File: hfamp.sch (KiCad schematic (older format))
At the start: 20 parts, among them K1 CONN_3, P1 CONN_2, Q1 DARL_N, U1 7805

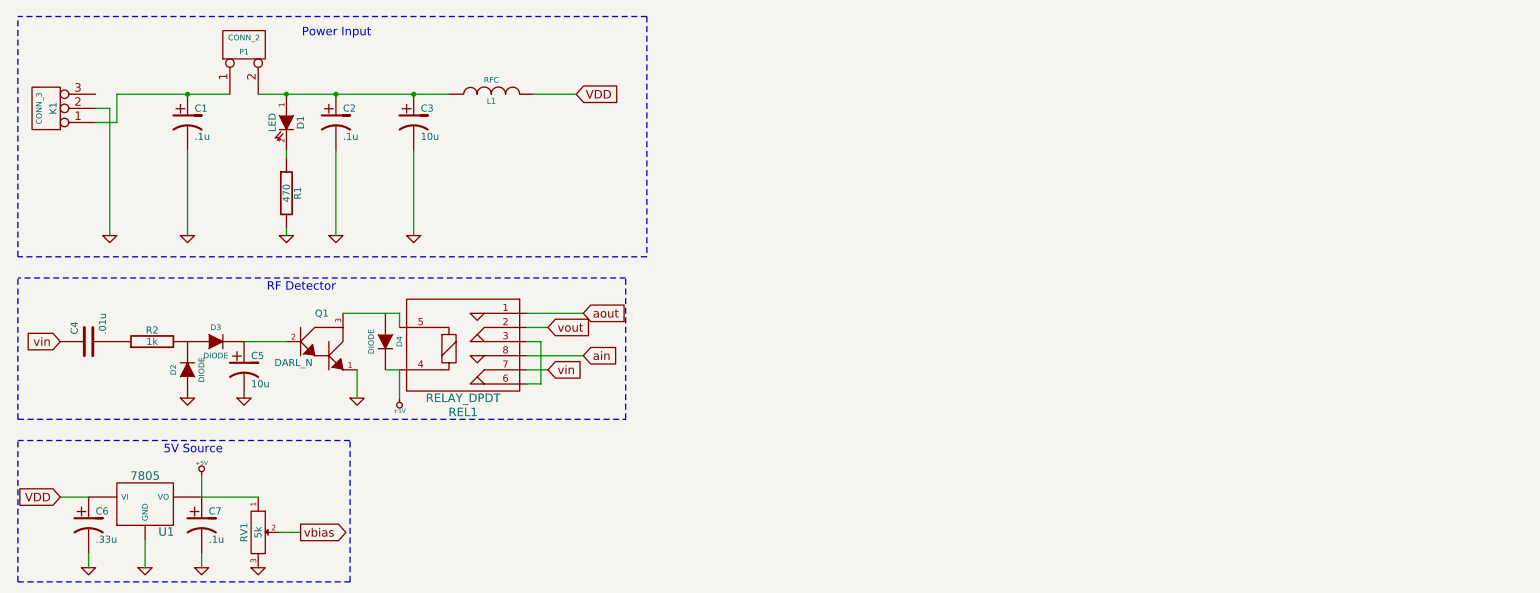
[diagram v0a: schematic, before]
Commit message: Finished schematic.
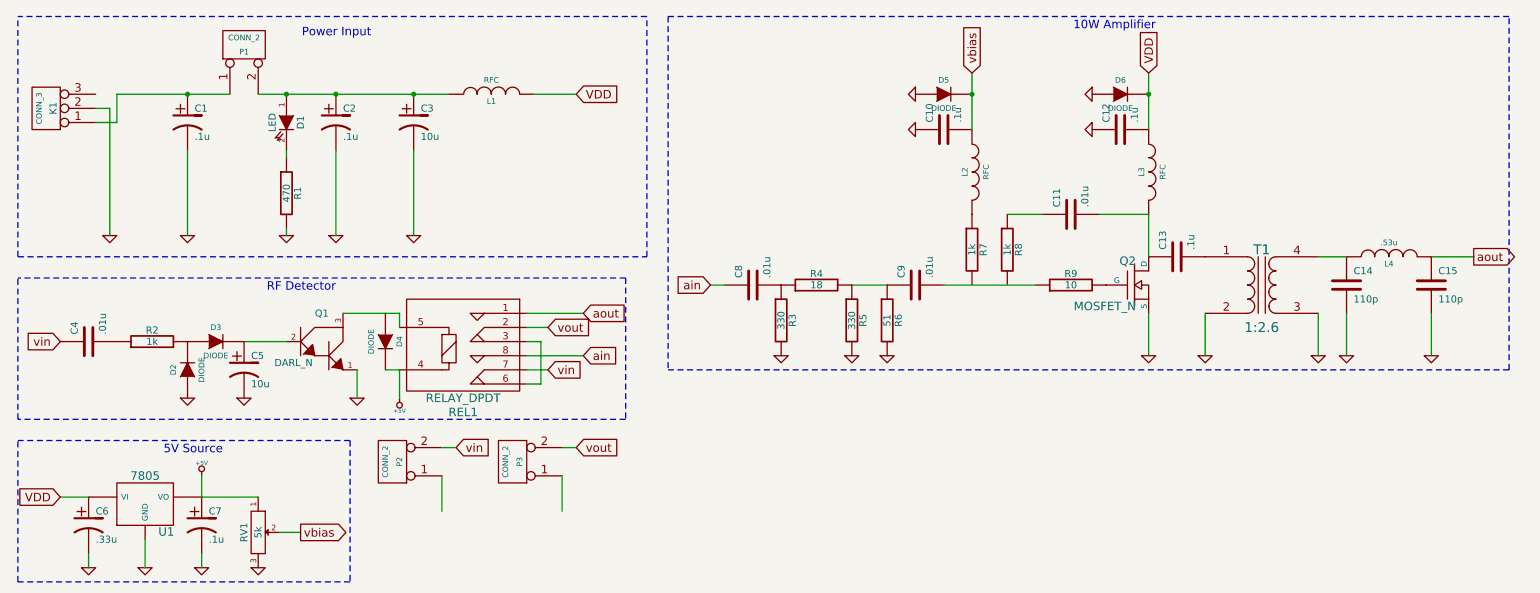
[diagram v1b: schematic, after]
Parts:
- added C10, C12, C13: .1u, symbol C
- added C11, C8, C9: .01u, symbol C
- added C14, C15: 110p, symbol C
- added D5, D6: DIODE, symbol DIODE
- added L2, L3: RFC, symbol INDUCTOR
- added L4: .53u, symbol INDUCTOR
- added P2, P3: CONN_2, symbol CONN_2
- added Q2: MOSFET_N, symbol MOSFET_N
- added R3, R5: 330, symbol R
- added R4: 18, symbol R
- added R6: 51, symbol R
- added R7, R8: 1k, symbol R
- added R9: 10, symbol R
- added T1: 1:2.6, symbol TRANSFO
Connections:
- wire segments 32 -> 51
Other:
- note added: "10W Amplifier"
